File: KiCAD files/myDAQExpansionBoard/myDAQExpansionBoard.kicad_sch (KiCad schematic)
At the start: 58 parts, among them J1 OSTV7XX3151, J2 Conn_01x05_Male, J3 Conn_01x05_Male, J4 Screw_Terminal_01x02, J5 Screw_Terminal_01x02, J6 Screw_Terminal_01x02, J7 Screw_Terminal_01x02, SW1 SW_Push, SW2 SW_Push, SW3 SW_SPST, SW4 SW_SPST, U1 74LS47, U2 HDSP-7501, U3 ACS712xLCTR-05B, U4 LM35-D, U5 L293D

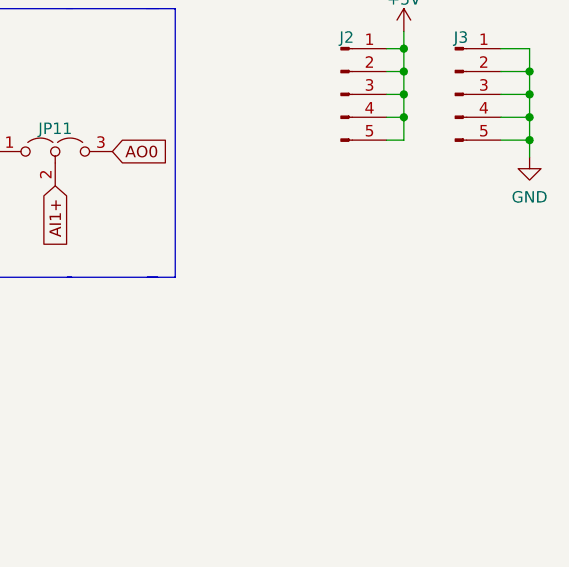
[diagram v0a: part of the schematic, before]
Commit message: Update myDAQExpansionBoard.kicad_sch
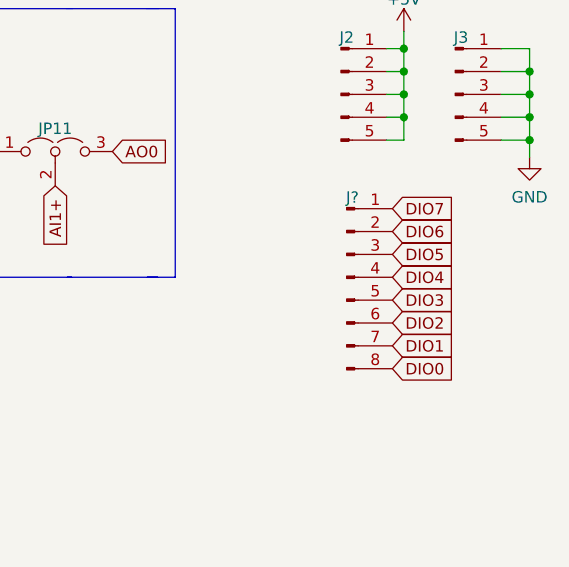
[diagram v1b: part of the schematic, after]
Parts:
- added J?: Conn_01x08_Male, symbol Connector:Conn_01x08_Male
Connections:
- net DIO0: now also J?.8 (Pin_8)
- net DIO1: now also J?.7 (Pin_7)
- net DIO2: now also J?.6 (Pin_6)
- net DIO3: now also J?.5 (Pin_5)
- net DIO4: now also J?.4 (Pin_4)
- net DIO5: now also J?.3 (Pin_3)
- net DIO6: now also J?.2 (Pin_2)
- net DIO7: now also J?.1 (Pin_1)
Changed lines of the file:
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@@
+    )
+  )
+  (global_label "DIO7" (shape input) (at 247.65 132.08 0) (fields_autoplaced)
+    (effects (font (size 1.27 1.27)) (justify left))
+    (property "Intersheet References" "${INTERSHEET_REFS}" (id 0) (at 254.4779 132.0006 0)
+      (effects (font (size 1.27 1.27)) (justify left) hide)
+    )
+  )
+  (global_label "DIO2" (shape input) (at 247.65 144.78 0) (fields_autoplaced)
+    (effects (font (size 1.27 1.27)) (justify left))
+    (property "Intersheet References" "${INTERSHEET_REFS}" (id 0) (at 254.4779 144.7006 0)
+      (effects (font (size 1.27 1.27)) (justify left) hide)
     )
   )
@@
     )
   )
+  (global_label "DIO0" (shape input) (at 247.65 149.86 0) (fields_autoplaced)
+    (effects (font (size 1.27 1.27)) (justify left))
+    (property "Intersheet References" "${INTERSHEET_REFS}" (id 0) (at 254.4779 149.7806 0)
+      (effects (font (size 1.27 1.27)) (justify left) hide)
+    )
+  )
   (global_label "DIO2" (shape input) (at 193.675 54.61 180) (fields_autoplaced)
     (effects (font (size 1.27 1.27)) (justify right))
@@
     )
   )
+  (global_label "DIO4" (shape input) (at 247.65 139.7 0) (fields_autoplaced)
+    (effects (font (size 1.27 1.27)) (justify left))
+    (property "Intersheet References" "${INTERSHEET_REFS}" (id 0) (at 254.4779 139.6206 0)
+      (effects (font (size 1.27 1.27)) (justify left) hide)
+    )
+  )
   (global_label "DIO4" (shape input) (at 31.75 55.88 0) (fields_autoplaced)
     (effects (font (size 1.27 1.27)) (justify left))
@@
     )
   )
+  (global_label "DIO1" (shape input) (at 247.65 147.32 0) (fields_autoplaced)
+    (effects (font (size 1.27 1.27)) (justify left))
+    (property "Intersheet References" "${INTERSHEET_REFS}" (id 0) (at 254.4779 147.2406 0)
+      (effects (font (size 1.27 1.27)) (justify left) hide)
+    )
+  )
   (global_label "DIO6" (shape input) (at 128.905 49.53 180) (fields_autoplaced)
     (effects (font (size 1.27 1.27)) (justify right))
@@
     )
   )
+  (global_label "DIO5" (shape input) (at 247.65 137.16 0) (fields_autoplaced)
+    (effects (font (size 1.27 1.27)) (justify left))
+    (property "Intersheet References" "${INTERSHEET_REFS}" (id 0) (at 254.4779 137.0806 0)
+      (effects (font (size 1.27 1.27)) (justify left) hide)
+    )
+  )
+  (global_label "DIO6" (shape input) (at 247.65 134.62 0) (fields_autoplaced)
+    (effects (font (size 1.27 1.27)) (justify left))
+    (property "Intersheet References" "${INTERSHEET_REFS}" (id 0) (at 254.4779 134.5406 0)
+      (effects (font (size 1.27 1.27)) (justify left) hide)
+    )
+  )
   (global_label "DIO2" (shape input) (at 83.82 76.835 180) (fields_autoplaced)
     (effects (font (size 1.27 1.27)) (justify right))
     (property "Intersheet References" "${INTERSHEET_REFS}" (id 0) (at 76.9921 76.7556 0)
       (effects (font (size 1.27 1.27)) (justify right) hide)
+    )
+  )
+  (global_label "DIO3" (shape input) (at 247.65 142.24 0) (fields_autoplaced)
+    (effects (font (size 1.27 1.27)) (justify left))
+    (property "Intersheet References" "${INTERSHEET_REFS}" (id 0) (at 254.4779 142.1606 0)
+      (effects (font (size 1.27 1.27)) (justify left) hide)
     )
   )
@@
     (pin "2")
   )
+  (symbol (lib_id "Connector:Conn_01x08_Male") (at 242.57 139.7 0) (unit 1)
+    (in_bom yes) (on_board yes) (fields_autoplaced)
+    (property "Reference" "J?" (id 0) (at 243.205 130.841 0))
+    (property "Value" "Conn_01x08_Male" (id 1) (at 243.205 130.8409 0)
+      (effects (font (size 1.27 1.27)) hide)
+    )
+    (property "Footprint" "" (id 2) (at 242.57 139.7 0)
+      (effects (font (size 1.27 1.27)) hide)
+    )
+    (property "Datasheet" "~" (id 3) (at 242.57 139.7 0)
+      (effects (font (size 1.27 1.27)) hide)
+    )
+    (pin "1")
+    (pin "2")
+    (pin "3")
+    (pin "4")
+    (pin "5")
+    (pin "6")
+    (pin "7")
+    (pin "8")
+  )
   (symbol (lib_id "Device:R") (at 122.555 88.265 90) (unit 1)
     (in_bom yes) (on_board yes)
@@
       (reference "J7") (unit 1) (value "Screw_Terminal_01x02") (footprint "")
     )
+    (path "/e978b021-68a3-493c-9c98-1e7ae8b7e007"
+      (reference "J?") (unit 1) (value "Conn_01x08_Male") (footprint "")
+    )
     (path "/79d1d2fe-44ad-4ea6-a4d2-2be9874caeed"
